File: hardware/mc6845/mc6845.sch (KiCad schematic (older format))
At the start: 11 parts, among them J1 Conn_02x20_Odd_Even, U1 MC6845, U10 AT28C16, U11 74LS32, U12 74LS163, U13 74LS04, U14 74LS08, U15 74LS74, U16 74LS174, U17 74LS165, X1 25.175MHz

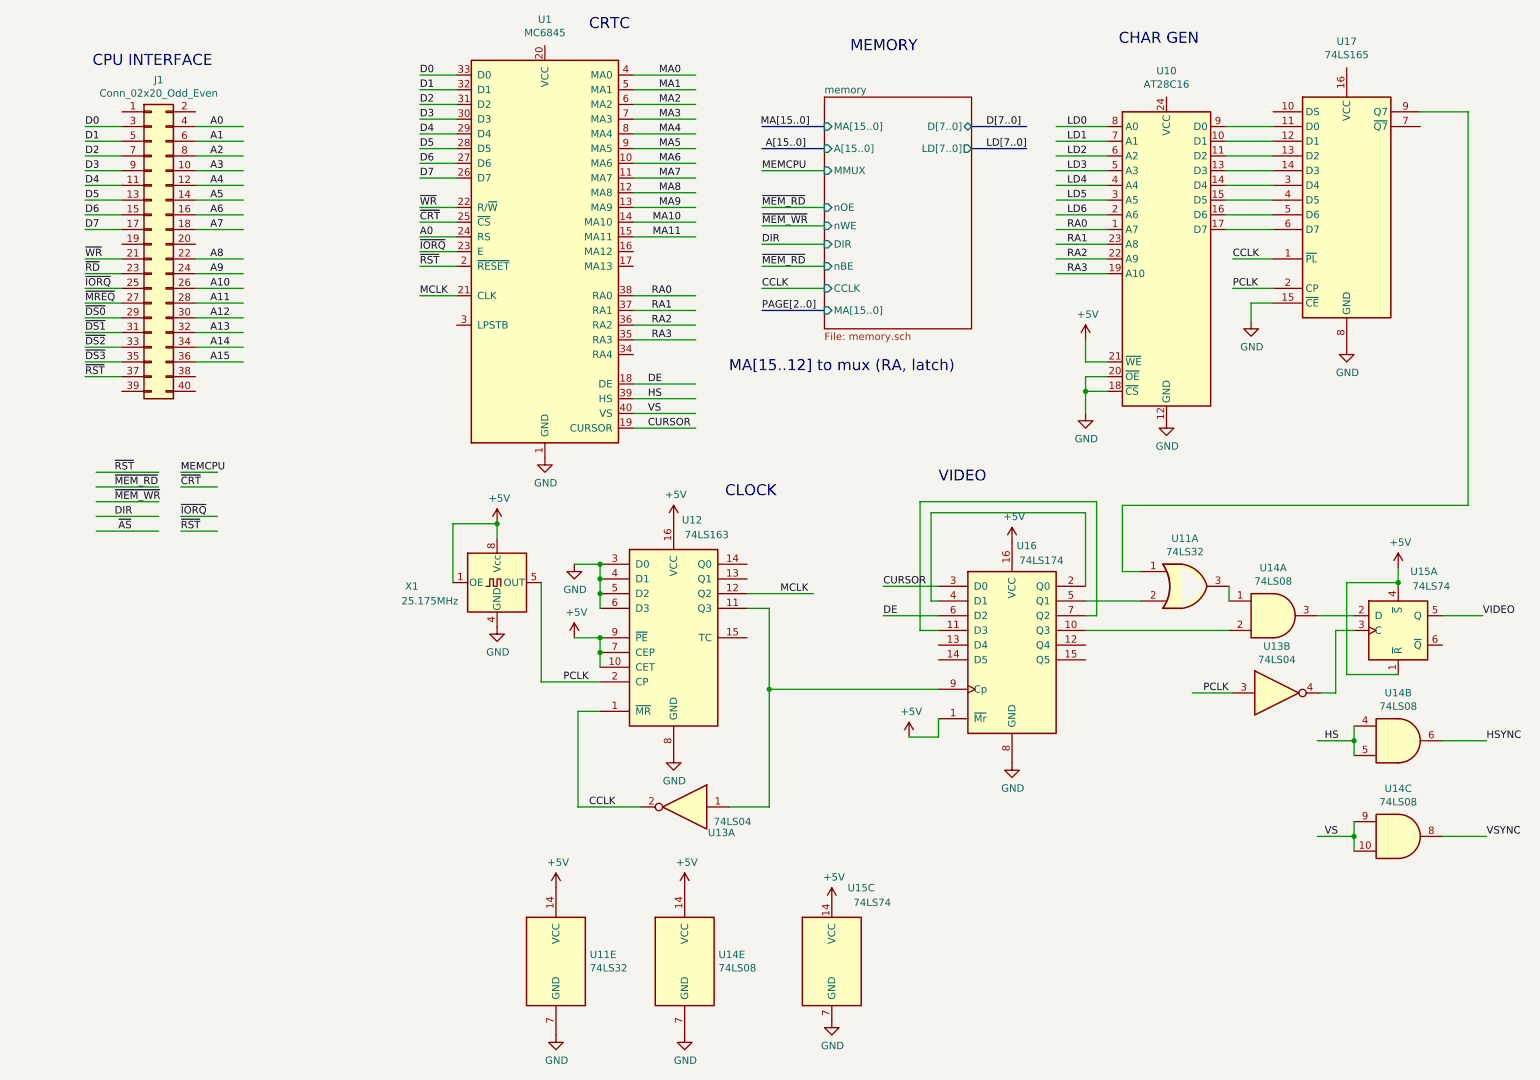
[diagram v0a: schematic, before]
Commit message: memory wiring
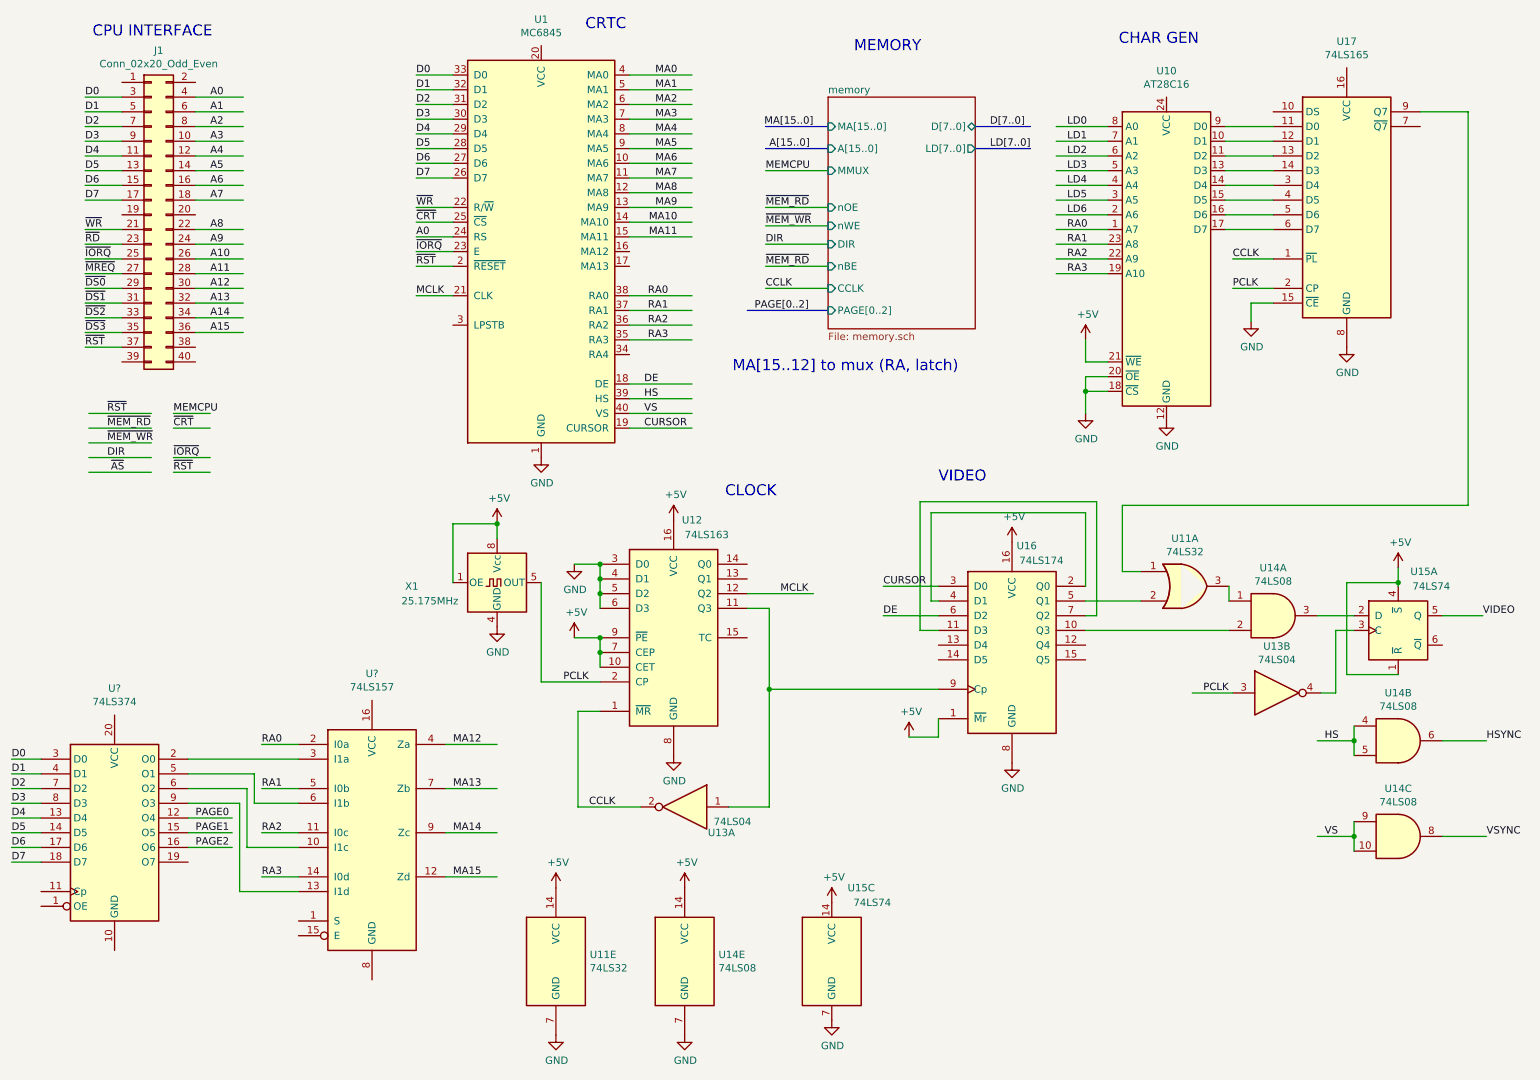
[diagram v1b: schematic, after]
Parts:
- added U?: 74LS157, symbol 74xx:74LS157
- added U?: 74LS374, symbol 74xx:74LS374
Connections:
- net labels added: MA12, MA13, MA14, MA15, PAGE0, PAGE1, PAGE2, PAGE[0..2]
- net labels removed: PAGE[2..0]
- wire segments 172 -> 201
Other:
- moved on the sheet: J1, U1
